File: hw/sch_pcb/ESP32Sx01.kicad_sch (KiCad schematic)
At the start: 37 parts, among them J1 HEADER_1x03, J2 USBC_USB4105-GF-A, J3 HEADER_1x12, J4 HEADER_1x12, J5 HEADER_1x12, J6 HEADER_1x03, J7 HEADER_2x05, Q1 BC817-25, SW1 434133025816, SW2 434133025816, U1 NCP1117-3.3, U2 USBLC6-2SC6, U3 ESP32-S3-MINI-1, Y1 Crystal_Small

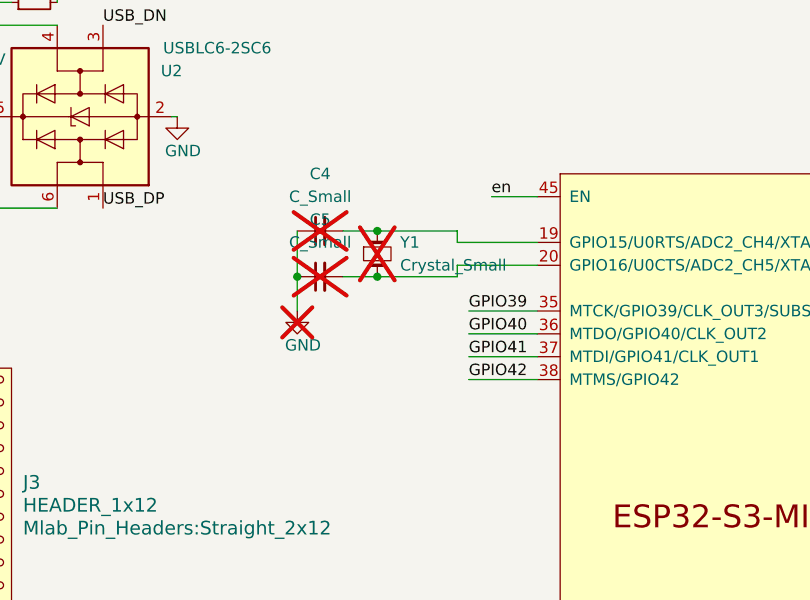
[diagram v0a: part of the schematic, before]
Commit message: Update UST_IDs.
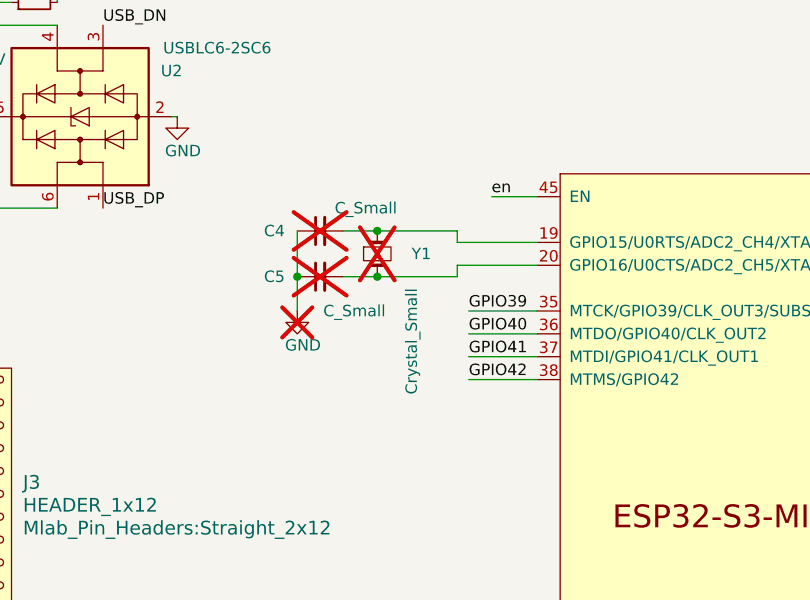
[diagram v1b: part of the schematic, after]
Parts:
- C1, C6, C7: UST_ID (none) -> 5c70984712875079b91f8b4c
- C2, C3, C8: UST_ID (none) -> 5c70984712875079b91f8b53
- C4, C5, Y1: now left out of the parts list
- D1: UST_ID (none) -> 60879d38128750769ee58e48
- D2: UST_ID (none) -> 650b35ab462c6d9e720543d0
- J2: UST_ID (none) -> 5fa0f94612875025b397795e
- Q1: UST_ID (none) -> 5c70984712875079b91f8aea
- R1, R2: UST_ID (none) -> 5fa0fc3e12875025b3977997
- R3, R4: UST_ID (none) -> 5c70984512875079b91f898c
- R5, R6: UST_ID (none) -> 5c70984512875079b91f897d
- R7: UST_ID (none) -> 5fa12b6012875025b3977a16
- SW1, SW2: UST_ID (none) -> 6998c49ed42e6e3c4d330f22
- U1: UST_ID (none) -> 5c70984712875079b91f8af9
- U2: UST_ID (none) -> 5e82e0691287502a334a778c
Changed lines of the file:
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@@
 			)
 		)
+		(property "UST_ID" "5fa0fc3e12875025b3977997"
+			(at 58.42 59.69 90)
+			(effects
+				(font
+					(size 1.27 1.27)
+				)
+				(hide yes)
+			)
+		)
 		(pin "1"
 		)
@@
 		(unit 1)
 		(exclude_from_sim no)
-		(in_bom yes)
+		(in_bom no)
 		(on_board yes)
 		(dnp yes)
-		(fields_autoplaced yes)
 		(property "Reference" "C5"
-			(at 90.1763 83.82 90)
+			(at 85.09 90.17 90)
 			(effects
 				(font
@@
 		)
 		(property "Value" "C_Small"
-			(at 90.1763 86.36 90)
+			(at 93.98 93.98 90)
 			(effects
 				(font
@@
 			)
 		)
+		(property "UST_ID" "5c70984512875079b91f898c"
+			(at 125.73 26.67 0)
+			(effects
+				(font
+					(size 1.27 1.27)
+				)
+				(hide yes)
+			)
+		)
 		(pin "1"
 		)
@@
 			)
 		)
+		(property "UST_ID" "650b35ab462c6d9e720543d0"
+			(at 81.28 31.75 90)
+			(effects
+				(font
+					(size 1.27 1.27)
+				)
+				(hide yes)
+			)
+		)
 		(pin "1"
 		)
@@
 			)
 		)
+		(property "UST_ID" "6998c49ed42e6e3c4d330f22"
+			(at 120.65 31.75 0)
+			(effects
+				(font
+					(size 1.27 1.27)
+				)
+				(hide yes)
+			)
+		)
 		(pin "1"
 		)
@@
 			)
 		)
+		(property "UST_ID" "5c70984712875079b91f8af9"
+			(at 63.5 26.67 0)
+			(effects
+				(font
+					(size 1.27 1.27)
+				)
+				(hide yes)
+			)
+		)
 		(pin "1"
 		)
@@
 			)
 		)
+		(property "UST_ID" "5c70984712875079b91f8b53"
+			(at 168.91 31.75 0)
+			(effects
+				(font
+					(size 1.27 1.27)
+				)
+				(hide yes)
+			)
+		)
 		(pin "1"
 		)
@@
 			)
 		)
+		(property "UST_ID" "5c70984512875079b91f898c"
+			(at 149.86 26.67 0)
+			(effects
+				(font
+					(size 1.27 1.27)
+				)
+				(hide yes)
+			)
+		)
 		(pin "1"
 		)
@@
 			)
 		)
+		(property "UST_ID" "5c70984712875079b91f8b53"
+			(at 53.34 29.21 0)
+			(effects
+				(font
+					(size 1.27 1.27)
+				)
+				(hide yes)
+			)
+		)
 		(pin "1"
 		)
@@
 			)
 		)
+		(property "UST_ID" "5c70984712875079b91f8b4c"
+			(at 44.45 29.21 0)
+			(effects
+				(font
+					(size 1.27 1.27)
+				)
+				(hide yes)
+			)
+		)
 		(pin "1"
 		)
@@
 			)
 		)
+		(property "UST_ID" "5c70984512875079b91f897d"
+			(at 264.16 64.77 90)
+			(effects
+				(font
+					(size 1.27 1.27)
+				)
+				(hide yes)
+			)
+		)
 		(pin "1"
 		)
@@
 			)
 		)
+		(property "UST_ID" "5c70984712875079b91f8b4c"
+			(at 149.86 34.29 0)
+			(effects
+				(font
+					(size 1.27 1.27)
+				)
+				(hide yes)
+			)
+		)
 		(pin "1"
 		)
@@
 			)
 		)
+		(property "UST_ID" "5c70984512875079b91f897d"
+			(at 242.57 58.42 0)
+			(effects
+				(font
+					(size 1.27 1.27)
+				)
+				(hide yes)
+			)
+		)
 		(pin "1"
 		)
@@
 		(unit 1)
 		(exclude_from_sim no)
-		(in_bom yes)
+		(in_bom no)
 		(on_board yes)
 		(dnp yes)
-		(fields_autoplaced yes)
 		(property "Reference" "Y1"
-			(at 99.06 86.3599 90)
+			(at 100.33 87.63 90)
 			(effects
 				(font
@@
 		)
 		(property "Value" "Crystal_Small"
-			(at 99.06 88.8999 90)
+			(at 100.33 91.44 0)
 			(effects
 				(font
@@
 			)
 		)
+		(property "UST_ID" "5fa12b6012875025b3977a16"
+			(at 274.32 57.15 0)
+			(effects
+				(font
+					(size 1.27 1.27)
+				)
+				(hide yes)
+			)
+		)
 		(pin "1"
 		)
@@
 			)
 		)
+		(property "UST_ID" "5e82e0691287502a334a778c"
+			(at 63.5 72.39 90)
+			(effects
+				(font
+					(size 1.27 1.27)
+				)
+				(hide yes)
+			)
+		)
 		(pin "1"
 		)
@@
 			)
 		)
+		(property "UST_ID" "5c70984712875079b91f8b4c"
+			(at 125.73 34.29 0)
+			(effects
+				(font
+					(size 1.27 1.27)
+				)
+				(hide yes)
+			)
+		)
 		(pin "1"
 		)
@@
 			)
 		)
+		(property "UST_ID" "5c70984712875079b91f8b53"
+			(at 73.66 31.75 0)
+			(effects
+				(font
+					(size 1.27 1.27)
+				)
+				(hide yes)
+			)
+		)
 		(pin "1"
 		)
@@
 			)
 		)
+		(property "UST_ID" "5c70984712875079b91f8aea"
+			(at 271.78 64.77 0)
+			(effects
+				(font
+					(size 1.27 1.27)
+				)
+				(hide yes)
+			)
+		)
 		(pin "1"
 		)
@@
 		(unit 1)
 		(exclude_from_sim no)
-		(in_bom yes)
+		(in_bom no)
 		(on_board yes)
 		(dnp yes)
-		(fields_autoplaced yes)
 		(property "Reference" "C4"
-			(at 90.1763 78.74 90)
+			(at 85.09 85.09 90)
 			(effects
 				(font
@@
 		)
 		(property "Value" "C_Small"
-			(at 90.1763 81.28 90)
+			(at 95.25 82.55 90)
 			(effects
 				(font
@@
 			)
 		)
+		(property "UST_ID" "6998c49ed42e6e3c4d330f22"
+			(at 144.78 31.75 0)
+			(effects
+				(font
+					(size 1.27 1.27)
+				)
+				(hide yes)
+			)
+		)
 		(pin "1"
 		)
@@
 			)
 		)
+		(property "UST_ID" "5fa0f94612875025b397795e"
+			(at 34.29 67.31 0)
+			(effects
+				(font
+					(size 1.27 1.27)
+				)
+				(hide yes)
+			)
+		)
 		(pin "A1/B12"
 		)
@@
 			)
 		)
+		(property "UST_ID" "5fa0fc3e12875025b3977997"
+			(at 58.42 52.07 90)
+			(effects
+				(font
+					(size 1.27 1.27)
+				)
+				(hide yes)
+			)
+		)
 		(pin "1"
 		)
@@
 			(effects
 				(font
+					(size 1.27 1.27)
+				)
+				(hide yes)
+			)
+		)
+		(property "UST_ID" "60879d38128750769ee58e48"
+			(at 38.1 30.48 90)
+			(effects
+				(font
